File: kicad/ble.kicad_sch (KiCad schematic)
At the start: 12 parts, among them J10 Conn_Coaxial, U16 NRF52832-QFAA-R, Y2 32MHz

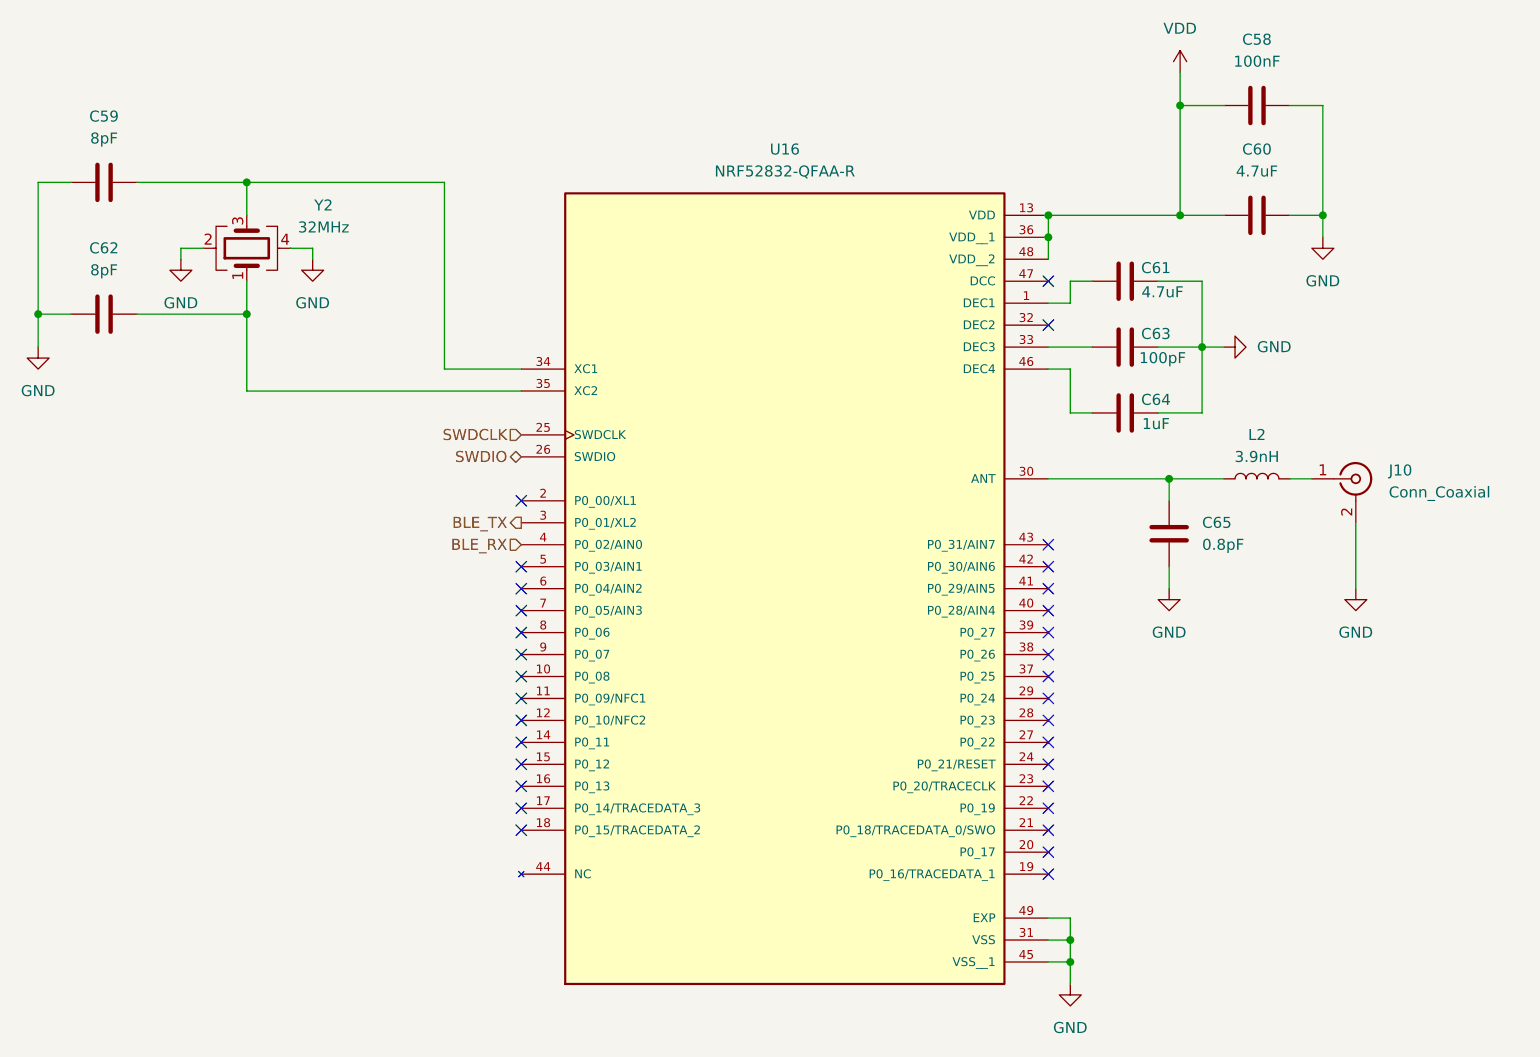
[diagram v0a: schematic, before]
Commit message: gate driver mostly schematic'd and pcb started
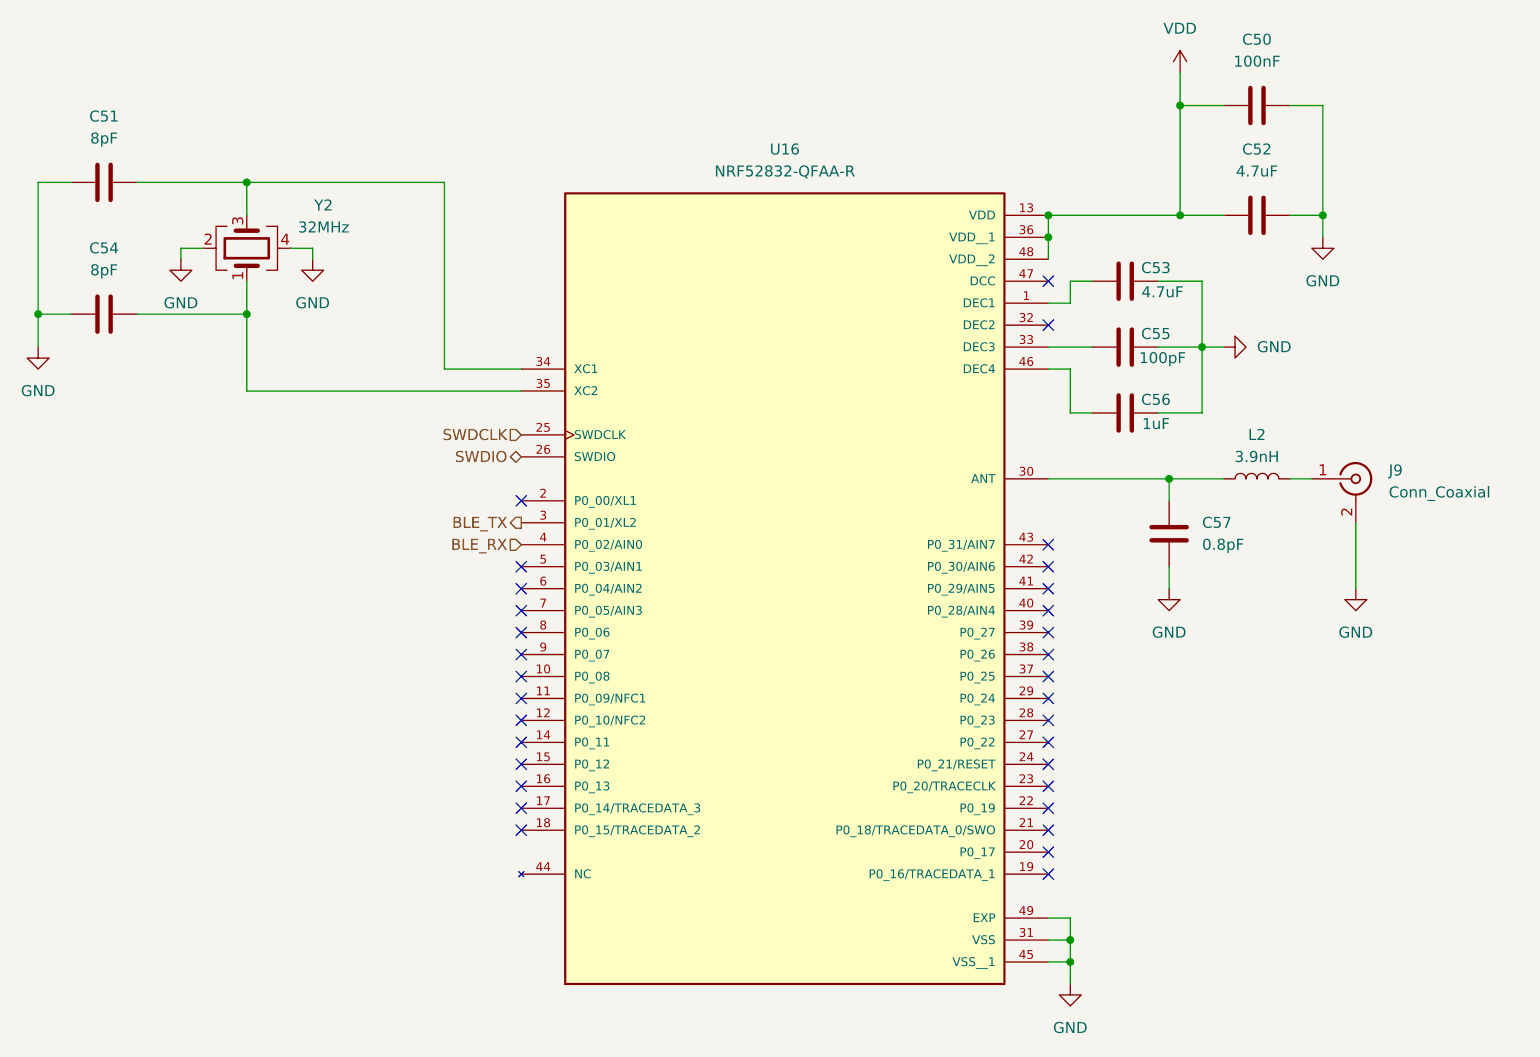
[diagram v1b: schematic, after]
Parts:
- renumbered C58 to C50, C59 to C51, C60 to C52, C61 to C53, C62 to C54, C63 to C55, C64 to C56, C65 to C57, J10 to J9
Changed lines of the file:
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@@
 		(dnp no)
 		(fields_autoplaced yes)
-		(property "Reference" "J10"
+		(property "Reference" "J9"
 			(at 209.55 79.0331 0)
 			(effects
@@
 			(project ""
 				(path "/83aea3b7-5b9b-498e-8d41-e84fae2f87fa/7fcb459e-6347-48a4-bd99-c80bd89cbe59"
-					(reference "J10")
+					(reference "J9")
 					(unit 1)
 				)
@@
 		(dnp no)
 		(fields_autoplaced yes)
-		(property "Reference" "#PWR098"
+		(property "Reference" "#PWR085"
 			(at 205.74 99.06 0)
 			(effects
@@
 			(project "resc"
 				(path "/83aea3b7-5b9b-498e-8d41-e84fae2f87fa/7fcb459e-6347-48a4-bd99-c80bd89cbe59"
-					(reference "#PWR098")
+					(reference "#PWR085")
 					(unit 1)
 				)
@@
 		(on_board yes)
 		(dnp no)
-		(property "Reference" "C61"
+		(property "Reference" "C53"
 			(at 182.626 55.626 90)
 			(effects
@@
 			(project "resc"
 				(path "/83aea3b7-5b9b-498e-8d41-e84fae2f87fa/7fcb459e-6347-48a4-bd99-c80bd89cbe59"
-					(reference "C61")
+					(reference "C53")
 					(unit 1)
 				)
@@
 		(on_board yes)
 		(dnp no)
-		(property "Reference" "#PWR094"
+		(property "Reference" "#PWR081"
 			(at 85.09 60.96 0)
 			(effects
@@
 			(project "resc"
 				(path "/83aea3b7-5b9b-498e-8d41-e84fae2f87fa/7fcb459e-6347-48a4-bd99-c80bd89cbe59"
-					(reference "#PWR094")
+					(reference "#PWR081")
 					(unit 1)
 				)
@@
 		(on_board yes)
 		(dnp no)
-		(property "Reference" "C64"
+		(property "Reference" "C56"
 			(at 182.626 70.866 90)
 			(effects
@@
 			(project "resc"
 				(path "/83aea3b7-5b9b-498e-8d41-e84fae2f87fa/7fcb459e-6347-48a4-bd99-c80bd89cbe59"
-					(reference "C64")
+					(reference "C56")
 					(unit 1)
 				)
@@
 		(on_board yes)
 		(dnp no)
-		(property "Reference" "C63"
+		(property "Reference" "C55"
 			(at 182.626 63.246 90)
 			(effects
@@
 			(project "resc"
 				(path "/83aea3b7-5b9b-498e-8d41-e84fae2f87fa/7fcb459e-6347-48a4-bd99-c80bd89cbe59"
-					(reference "C63")
+					(reference "C55")
 					(unit 1)
 				)
@@
 		(dnp no)
 		(fields_autoplaced yes)
-		(property "Reference" "#PWR099"
+		(property "Reference" "#PWR086"
 			(at 172.72 144.78 0)
 			(effects
@@
 			(project ""
 				(path "/83aea3b7-5b9b-498e-8d41-e84fae2f87fa/7fcb459e-6347-48a4-bd99-c80bd89cbe59"
-					(reference "#PWR099")
+					(reference "#PWR086")
 					(unit 1)
 				)
@@
 		(on_board yes)
 		(dnp no)
-		(property "Reference" "#PWR093"
+		(property "Reference" "#PWR080"
 			(at 69.85 60.96 0)
 			(effects
@@
 			(project "resc"
 				(path "/83aea3b7-5b9b-498e-8d41-e84fae2f87fa/7fcb459e-6347-48a4-bd99-c80bd89cbe59"
-					(reference "#PWR093")
+					(reference "#PWR080")
 					(unit 1)
 				)
@@
 		(dnp no)
 		(fields_autoplaced yes)
-		(property "Reference" "#PWR091"
+		(property "Reference" "#PWR078"
 			(at 185.42 36.83 0)
 			(effects
@@
 			(project ""
 				(path "/83aea3b7-5b9b-498e-8d41-e84fae2f87fa/7fcb459e-6347-48a4-bd99-c80bd89cbe59"
-					(reference "#PWR091")
+					(reference "#PWR078")
 					(unit 1)
 				)
@@
 		(dnp no)
 		(fields_autoplaced yes)
-		(property "Reference" "C58"
+		(property "Reference" "C50"
 			(at 194.31 29.21 90)
 			(effects
@@
 			(project "resc"
 				(path "/83aea3b7-5b9b-498e-8d41-e84fae2f87fa/7fcb459e-6347-48a4-bd99-c80bd89cbe59"
-					(reference "C58")
+					(reference "C50")
 					(unit 1)
 				)
@@
 		(dnp no)
 		(fields_autoplaced yes)
-		(property "Reference" "#PWR092"
+		(property "Reference" "#PWR079"
 			(at 201.93 58.42 0)
 			(effects
@@
 			(project ""
 				(path "/83aea3b7-5b9b-498e-8d41-e84fae2f87fa/7fcb459e-6347-48a4-bd99-c80bd89cbe59"
-					(reference "#PWR092")
+					(reference "#PWR079")
 					(unit 1)
 				)
@@
 		(dnp no)
 		(fields_autoplaced yes)
-		(property "Reference" "C60"
+		(property "Reference" "C52"
 			(at 194.31 41.91 90)
 			(effects
@@
 			(project ""
 				(path "/83aea3b7-5b9b-498e-8d41-e84fae2f87fa/7fcb459e-6347-48a4-bd99-c80bd89cbe59"
-					(reference "C60")
+					(reference "C52")
 					(unit 1)
 				)
@@
 		(dnp no)
 		(fields_autoplaced yes)
-		(property "Reference" "C65"
+		(property "Reference" "C57"
 			(at 187.96 85.0899 0)
 			(effects
@@
 			(project ""
 				(path "/83aea3b7-5b9b-498e-8d41-e84fae2f87fa/7fcb459e-6347-48a4-bd99-c80bd89cbe59"
-					(reference "C65")
+					(reference "C57")
 					(unit 1)
 				)
@@
 		(dnp no)
 		(fields_autoplaced yes)
-		(property "Reference" "#PWR096"
+		(property "Reference" "#PWR082"
 			(at 53.34 71.12 0)
 			(effects
@@
 			(project ""
 				(path "/83aea3b7-5b9b-498e-8d41-e84fae2f87fa/7fcb459e-6347-48a4-bd99-c80bd89cbe59"
-					(reference "#PWR096")
+					(reference "#PWR082")
 					(unit 1)
 				)
@@
 		(dnp no)
 		(fields_autoplaced yes)
-		(property "Reference" "C59"
+		(property "Reference" "C51"
 			(at 60.96 38.1 90)
 			(effects
@@
 			(project ""
 				(path "/83aea3b7-5b9b-498e-8d41-e84fae2f87fa/7fcb459e-6347-48a4-bd99-c80bd89cbe59"
-					(reference "C59")
+					(reference "C51")
 					(unit 1)
 				)
@@
 		(dnp no)
 		(fields_autoplaced yes)
-		(property "Reference" "#PWR097"
+		(property "Reference" "#PWR084"
 			(at 184.15 99.06 0)
 			(effects
@@
 			(project "resc"
 				(path "/83aea3b7-5b9b-498e-8d41-e84fae2f87fa/7fcb459e-6347-48a4-bd99-c80bd89cbe59"
-					(reference "#PWR097")
+					(reference "#PWR084")
 					(unit 1)
 				)
@@
 		(dnp no)
 		(fields_autoplaced yes)
-		(property "Reference" "#PWR095"
+		(property "Reference" "#PWR083"
 			(at 196.85 64.77 0)
 			(effects
@@
 			(project "resc"
 				(path "/83aea3b7-5b9b-498e-8d41-e84fae2f87fa/7fcb459e-6347-48a4-bd99-c80bd89cbe59"
-					(reference "#PWR095")
+					(reference "#PWR083")
 					(unit 1)
 				)
@@
 		(dnp no)
 		(fields_autoplaced yes)
-		(property "Reference" "C62"
+		(property "Reference" "C54"
 			(at 60.96 53.34 90)
 			(effects
@@
 			(project "resc"
 				(path "/83aea3b7-5b9b-498e-8d41-e84fae2f87fa/7fcb459e-6347-48a4-bd99-c80bd89cbe59"
-					(reference "C62")
-					(unit 1)
-				)
+					(reference "C54")
+					(unit 1)
+				)

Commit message: rev3 ordered
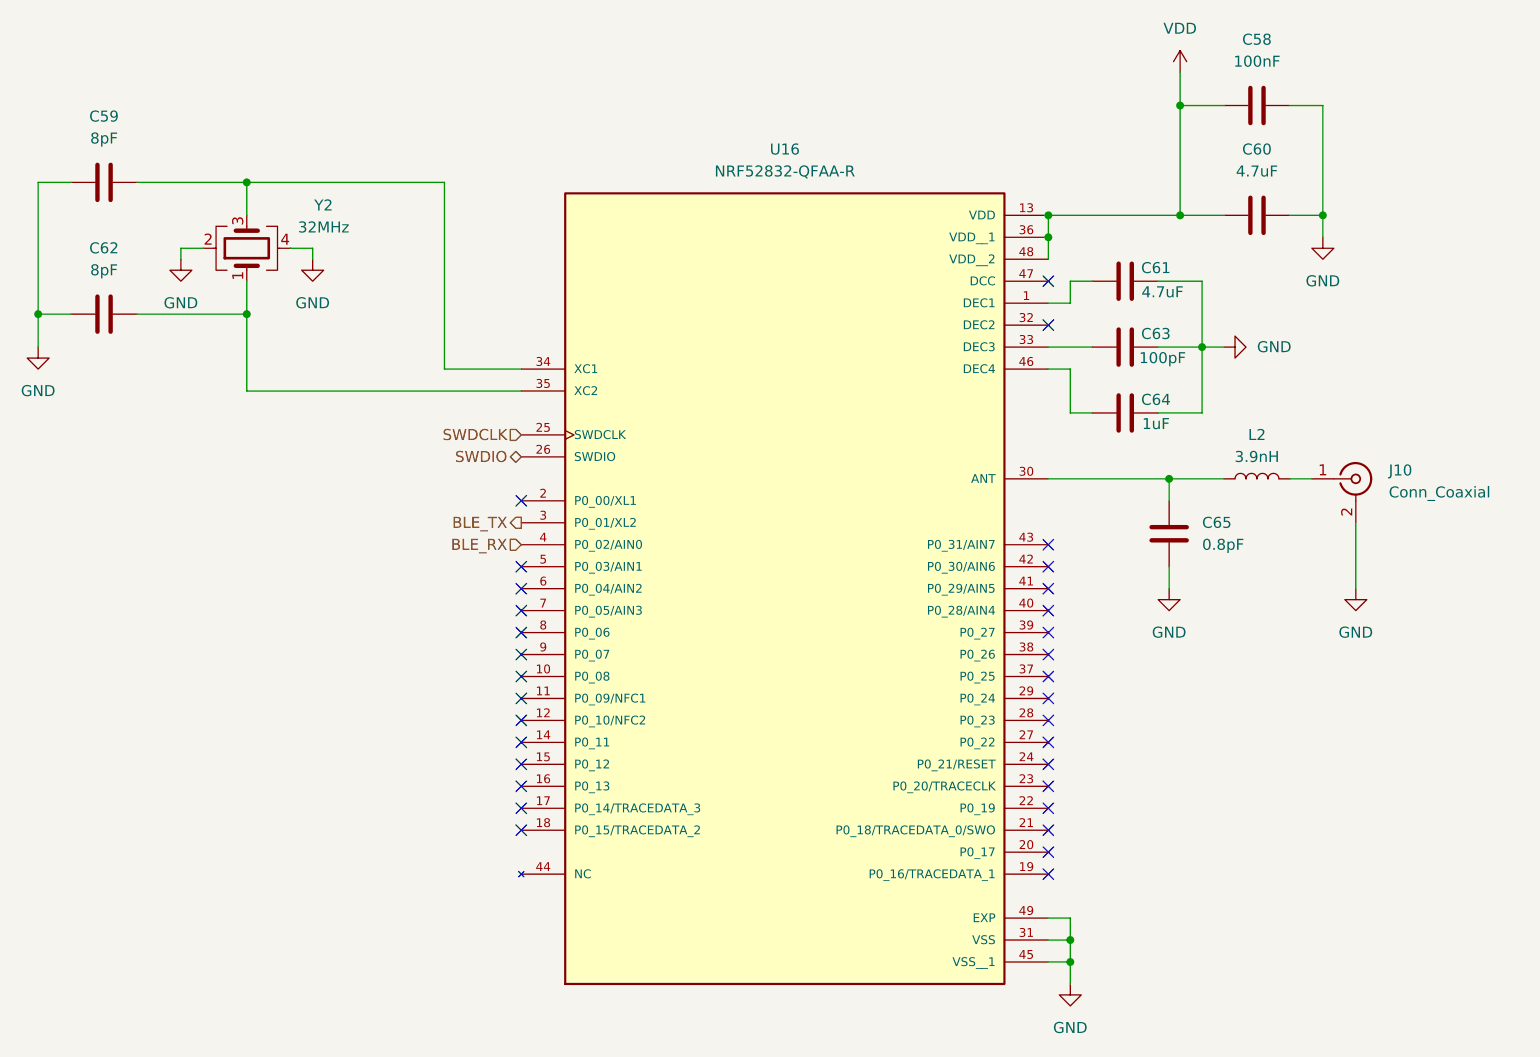
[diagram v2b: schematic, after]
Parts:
- renumbered C50 to C58, C51 to C59, C52 to C60, C53 to C61, C54 to C62, C55 to C63, C56 to C64, C57 to C65, J9 to J10
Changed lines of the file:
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@@
 		(dnp no)
 		(fields_autoplaced yes)
-		(property "Reference" "J9"
+		(property "Reference" "J10"
 			(at 209.55 79.0331 0)
 			(effects
@@
 			(project ""
 				(path "/83aea3b7-5b9b-498e-8d41-e84fae2f87fa/7fcb459e-6347-48a4-bd99-c80bd89cbe59"
-					(reference "J9")
+					(reference "J10")
 					(unit 1)
 				)
@@
 		(dnp no)
 		(fields_autoplaced yes)
-		(property "Reference" "#PWR085"
+		(property "Reference" "#PWR098"
 			(at 205.74 99.06 0)
 			(effects
@@
 			(project "resc"
 				(path "/83aea3b7-5b9b-498e-8d41-e84fae2f87fa/7fcb459e-6347-48a4-bd99-c80bd89cbe59"
-					(reference "#PWR085")
+					(reference "#PWR098")
 					(unit 1)
 				)
@@
 		(on_board yes)
 		(dnp no)
-		(property "Reference" "C53"
+		(property "Reference" "C61"
 			(at 182.626 55.626 90)
 			(effects
@@
 			(project "resc"
 				(path "/83aea3b7-5b9b-498e-8d41-e84fae2f87fa/7fcb459e-6347-48a4-bd99-c80bd89cbe59"
-					(reference "C53")
+					(reference "C61")
 					(unit 1)
 				)
@@
 		(on_board yes)
 		(dnp no)
-		(property "Reference" "#PWR081"
+		(property "Reference" "#PWR094"
 			(at 85.09 60.96 0)
 			(effects
@@
 			(project "resc"
 				(path "/83aea3b7-5b9b-498e-8d41-e84fae2f87fa/7fcb459e-6347-48a4-bd99-c80bd89cbe59"
-					(reference "#PWR081")
+					(reference "#PWR094")
 					(unit 1)
 				)
@@
 		(on_board yes)
 		(dnp no)
-		(property "Reference" "C56"
+		(property "Reference" "C64"
 			(at 182.626 70.866 90)
 			(effects
@@
 			(project "resc"
 				(path "/83aea3b7-5b9b-498e-8d41-e84fae2f87fa/7fcb459e-6347-48a4-bd99-c80bd89cbe59"
-					(reference "C56")
+					(reference "C64")
 					(unit 1)
 				)
@@
 		(on_board yes)
 		(dnp no)
-		(property "Reference" "C55"
+		(property "Reference" "C63"
 			(at 182.626 63.246 90)
 			(effects
@@
 			(project "resc"
 				(path "/83aea3b7-5b9b-498e-8d41-e84fae2f87fa/7fcb459e-6347-48a4-bd99-c80bd89cbe59"
-					(reference "C55")
+					(reference "C63")
 					(unit 1)
 				)
@@
 		(dnp no)
 		(fields_autoplaced yes)
-		(property "Reference" "#PWR086"
+		(property "Reference" "#PWR099"
 			(at 172.72 144.78 0)
 			(effects
@@
 			(project ""
 				(path "/83aea3b7-5b9b-498e-8d41-e84fae2f87fa/7fcb459e-6347-48a4-bd99-c80bd89cbe59"
-					(reference "#PWR086")
+					(reference "#PWR099")
 					(unit 1)
 				)
@@
 		(on_board yes)
 		(dnp no)
-		(property "Reference" "#PWR080"
+		(property "Reference" "#PWR093"
 			(at 69.85 60.96 0)
 			(effects
@@
 			(project "resc"
 				(path "/83aea3b7-5b9b-498e-8d41-e84fae2f87fa/7fcb459e-6347-48a4-bd99-c80bd89cbe59"
-					(reference "#PWR080")
+					(reference "#PWR093")
 					(unit 1)
 				)
@@
 		(dnp no)
 		(fields_autoplaced yes)
-		(property "Reference" "#PWR078"
+		(property "Reference" "#PWR091"
 			(at 185.42 36.83 0)
 			(effects
@@
 			(project ""
 				(path "/83aea3b7-5b9b-498e-8d41-e84fae2f87fa/7fcb459e-6347-48a4-bd99-c80bd89cbe59"
-					(reference "#PWR078")
+					(reference "#PWR091")
 					(unit 1)
 				)
@@
 		(dnp no)
 		(fields_autoplaced yes)
-		(property "Reference" "C50"
+		(property "Reference" "C58"
 			(at 194.31 29.21 90)
 			(effects
@@
 			(project "resc"
 				(path "/83aea3b7-5b9b-498e-8d41-e84fae2f87fa/7fcb459e-6347-48a4-bd99-c80bd89cbe59"
-					(reference "C50")
+					(reference "C58")
 					(unit 1)
 				)
@@
 		(dnp no)
 		(fields_autoplaced yes)
-		(property "Reference" "#PWR079"
+		(property "Reference" "#PWR092"
 			(at 201.93 58.42 0)
 			(effects
@@
 			(project ""
 				(path "/83aea3b7-5b9b-498e-8d41-e84fae2f87fa/7fcb459e-6347-48a4-bd99-c80bd89cbe59"
-					(reference "#PWR079")
+					(reference "#PWR092")
 					(unit 1)
 				)
@@
 		(dnp no)
 		(fields_autoplaced yes)
-		(property "Reference" "C52"
+		(property "Reference" "C60"
 			(at 194.31 41.91 90)
 			(effects
@@
 			(project ""
 				(path "/83aea3b7-5b9b-498e-8d41-e84fae2f87fa/7fcb459e-6347-48a4-bd99-c80bd89cbe59"
-					(reference "C52")
+					(reference "C60")
 					(unit 1)
 				)
@@
 		(dnp no)
 		(fields_autoplaced yes)
-		(property "Reference" "C57"
+		(property "Reference" "C65"
 			(at 187.96 85.0899 0)
 			(effects
@@
 			(project ""
 				(path "/83aea3b7-5b9b-498e-8d41-e84fae2f87fa/7fcb459e-6347-48a4-bd99-c80bd89cbe59"
-					(reference "C57")
+					(reference "C65")
 					(unit 1)
 				)
@@
 		(dnp no)
 		(fields_autoplaced yes)
-		(property "Reference" "#PWR082"
+		(property "Reference" "#PWR096"
 			(at 53.34 71.12 0)
 			(effects
@@
 			(project ""
 				(path "/83aea3b7-5b9b-498e-8d41-e84fae2f87fa/7fcb459e-6347-48a4-bd99-c80bd89cbe59"
-					(reference "#PWR082")
+					(reference "#PWR096")
 					(unit 1)
 				)
@@
 		(dnp no)
 		(fields_autoplaced yes)
-		(property "Reference" "C51"
+		(property "Reference" "C59"
 			(at 60.96 38.1 90)
 			(effects
@@
 			(project ""
 				(path "/83aea3b7-5b9b-498e-8d41-e84fae2f87fa/7fcb459e-6347-48a4-bd99-c80bd89cbe59"
-					(reference "C51")
+					(reference "C59")
 					(unit 1)
 				)
@@
 		(dnp no)
 		(fields_autoplaced yes)
-		(property "Reference" "#PWR084"
+		(property "Reference" "#PWR097"
 			(at 184.15 99.06 0)
 			(effects
@@
 			(project "resc"
 				(path "/83aea3b7-5b9b-498e-8d41-e84fae2f87fa/7fcb459e-6347-48a4-bd99-c80bd89cbe59"
-					(reference "#PWR084")
+					(reference "#PWR097")
 					(unit 1)
 				)
@@
 		(dnp no)
 		(fields_autoplaced yes)
-		(property "Reference" "#PWR083"
+		(property "Reference" "#PWR095"
 			(at 196.85 64.77 0)
 			(effects
@@
 			(project "resc"
 				(path "/83aea3b7-5b9b-498e-8d41-e84fae2f87fa/7fcb459e-6347-48a4-bd99-c80bd89cbe59"
-					(reference "#PWR083")
+					(reference "#PWR095")
 					(unit 1)
 				)
@@
 		(dnp no)
 		(fields_autoplaced yes)
-		(property "Reference" "C54"
+		(property "Reference" "C62"
 			(at 60.96 53.34 90)
 			(effects
@@
 			(project "resc"
 				(path "/83aea3b7-5b9b-498e-8d41-e84fae2f87fa/7fcb459e-6347-48a4-bd99-c80bd89cbe59"
-					(reference "C54")
-					(unit 1)
-				)
+					(reference "C62")
+					(unit 1)
+				)
